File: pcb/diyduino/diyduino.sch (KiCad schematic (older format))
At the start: 15 parts, among them U1 ATMEGA328-PU, U2 L7805, Y1 16MHz

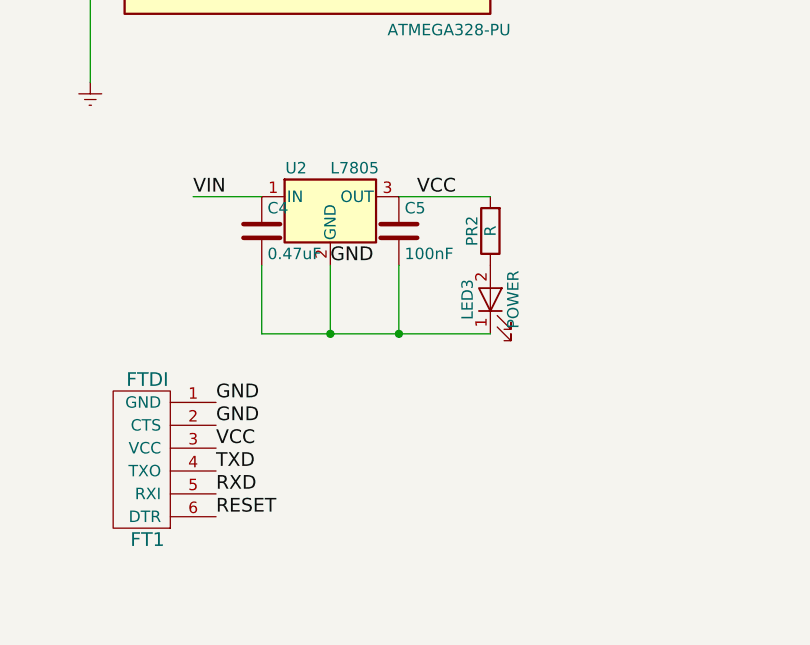
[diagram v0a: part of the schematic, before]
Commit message: Reworked diyduino module.
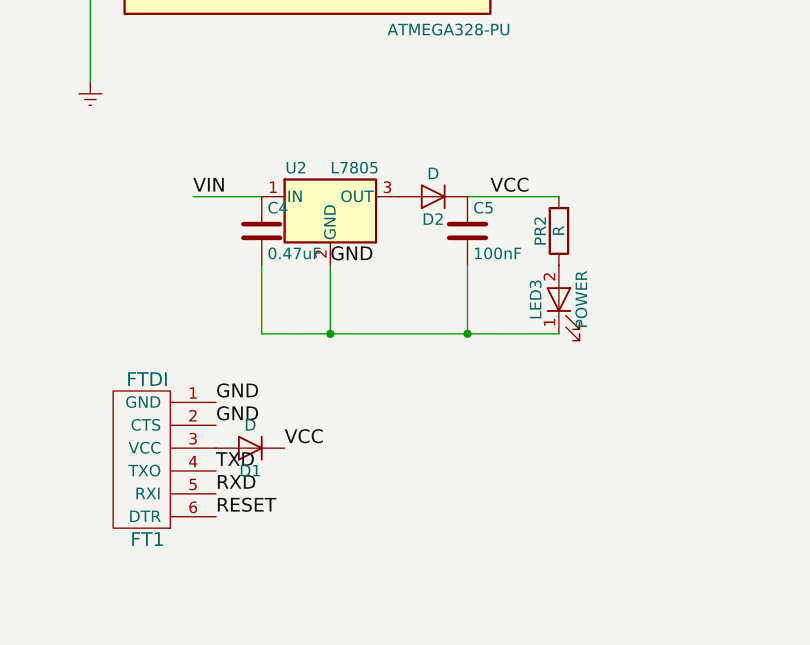
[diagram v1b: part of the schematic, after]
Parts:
- added D1, D2: D, Diodes_THT:D_T-1_P5.08mm_Horizontal, symbol D
- LED3: footprint LEDs:LED_D3.0mm -> LEDs:LED_Rectangular_W3.0mm_H2.0mm
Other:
- moved on the sheet: C5, LED3, PR2
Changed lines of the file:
@@
 L R PR2
 U 1 1 5AC0021E
-P 3500 4350
-F 0 "PR2" V 3580 4350 50  0000 C CNN
-F 1 "R" V 3500 4350 50  0000 C CNN
-F 2 "Resistors_THT:R_Axial_DIN0204_L3.6mm_D1.6mm_P7.62mm_Horizontal" V 3430 4350 50  0001 C CNN
-F 3 "" H 3500 4350 50  0001 C CNN
-	1    3500 4350
+P 3800 4350
+F 0 "PR2" V 3880 4350 50  0000 C CNN
+F 1 "R" V 3800 4350 50  0000 C CNN
+F 2 "Resistors_THT:R_Axial_DIN0204_L3.6mm_D1.6mm_P7.62mm_Horizontal" V 3730 4350 50  0001 C CNN
+F 3 "" H 3800 4350 50  0001 C CNN
+	1    3800 4350
 	-1   0    0    1
 $EndComp
@@
 L LED LED3
 U 1 1 5AC002AF
-P 3500 4650
-F 0 "LED3" H 3500 4750 50  0000 C CNN
-F 1 "POWER" H 3500 4550 50  0000 C CNN
-F 2 "LEDs:LED_D3.0mm" H 3500 4650 50  0001 C CNN
-F 3 "" H 3500 4650 50  0001 C CNN
-	1    3500 4650
+P 3800 4650
+F 0 "LED3" H 3800 4750 50  0000 C CNN
+F 1 "POWER" H 3800 4550 50  0000 C CNN
+F 2 "LEDs:LED_Rectangular_W3.0mm_H2.0mm" H 3800 4650 50  0001 C CNN
+F 3 "" H 3800 4650 50  0001 C CNN
+	1    3800 4650
 	0    -1   -1   0
 $EndComp
-Text Label 3350 4200 2    60   ~ 0
+Text Label 3500 4200 0    60   ~ 0
 VCC
 $Comp
@@
 Text Label 5350 5800 2    60   ~ 0
 A5
-Text Label 2300 5300 0    60   ~ 0
+Text Label 2600 5300 0    60   ~ 0
 VCC
 $Comp
@@
 L C C5
 U 1 1 5AC3FB72
-P 3100 4350
-F 0 "C5" H 3125 4450 50  0000 L CNN
-F 1 "100nF" H 3125 4250 50  0000 L CNN
-F 2 "Capacitors_THT:CP_Radial_D6.3mm_P2.50mm" H 3138 4200 50  0001 C CNN
-F 3 "" H 3100 4350 50  0001 C CNN
-	1    3100 4350
+P 3400 4350
+F 0 "C5" H 3425 4450 50  0000 L CNN
+F 1 "100nF" H 3425 4250 50  0000 L CNN
+F 2 "Capacitors_THT:CP_Radial_D6.3mm_P2.50mm" H 3438 4200 50  0001 C CNN
+F 3 "" H 3400 4350 50  0001 C CNN
+	1    3400 4350
 	1    0    0    -1
 $EndComp
@@
 	4200 1700 4200 1750
 Wire Wire Line
-	3100 4200 3500 4200
-Wire Wire Line
 	2800 4500 2800 4800
 Wire Wire Line
-	2500 4800 3500 4800
-Wire Wire Line
-	3100 4500 3100 4800
-Connection ~ 3100 4800
+	2500 4800 3800 4800
 Wire Wire Line
 	2500 4500 2500 4800
 Connection ~ 2800 4800
+$Comp
+L D D1
+U 1 1 5AC4FB56
+P 2450 5300
+F 0 "D1" H 2450 5400 50  0000 C CNN
+F 1 "D" H 2450 5200 50  0000 C CNN
+F 2 "Diodes_THT:D_T-1_P5.08mm_Horizontal" H 2450 5300 50  0001 C CNN
+F 3 "" H 2450 5300 50  0001 C CNN
+	1    2450 5300
+	-1   0    0    1
+$EndComp
+$Comp
+L D D2
+U 1 1 5AC4FCDF
+P 3250 4200
+F 0 "D2" H 3250 4300 50  0000 C CNN
+F 1 "D" H 3250 4100 50  0000 C CNN
+F 2 "Diodes_THT:D_T-1_P5.08mm_Horizontal" H 3250 4200 50  0001 C CNN
+F 3 "" H 3250 4200 50  0001 C CNN
+	1    3250 4200
+	-1   0    0    1
+$EndComp
+Wire Wire Line
+	3800 4200 3400 4200
+Wire Wire Line
+	3400 4500 3400 4800
+Connection ~ 3400 4800
 $EndSCHEMATC
